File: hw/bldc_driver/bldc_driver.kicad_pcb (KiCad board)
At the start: 2 copper layers, 127.5 x 96 mm, 131 parts, among them J1 430450412, J2 B4B-EH-A(LF)(SN), J3 B4B-EH-A(LF)(SN), J4 1733583, Q1 IRF540N, Q1 Q_NMOS_DGS, Q2 IRF540N, Q3 IRF540N, Q4 IRF540N, Q5 IRF540N, Q6 IRF540N, U1 CH32V30xRxTx, U10 TPS54202DDC, U11 AMC1200BDWV, U12 AMC1200BDWV, U13 AMC1200BDWV, U14 SN65HVD230, U2 STGAP2SCM, U3 STGAP2SCM, U4 STGAP2SCM, U5 STGAP2SCM, U6 STGAP2SCM, U7 STGAP2SCM, U8 TPS54202DDC, U9 AMC1200BDWV

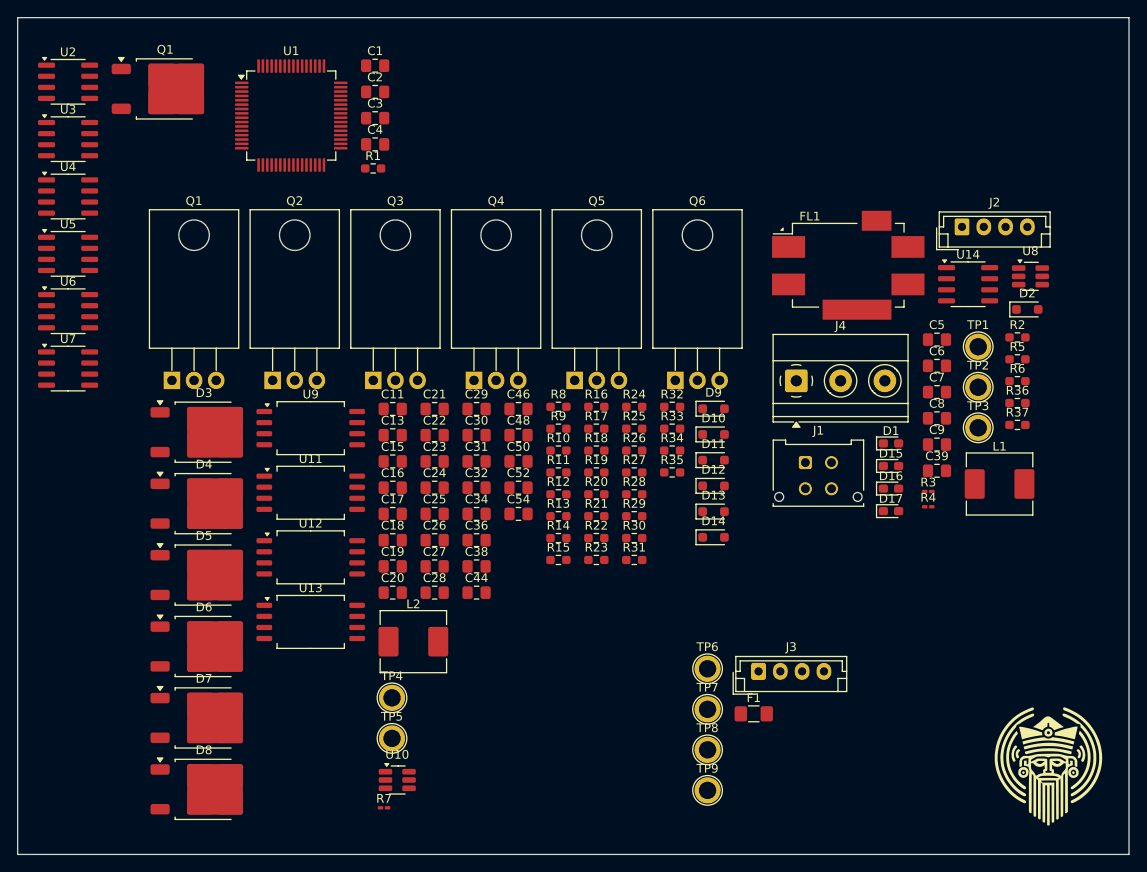
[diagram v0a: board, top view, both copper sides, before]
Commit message: bldc: start placement
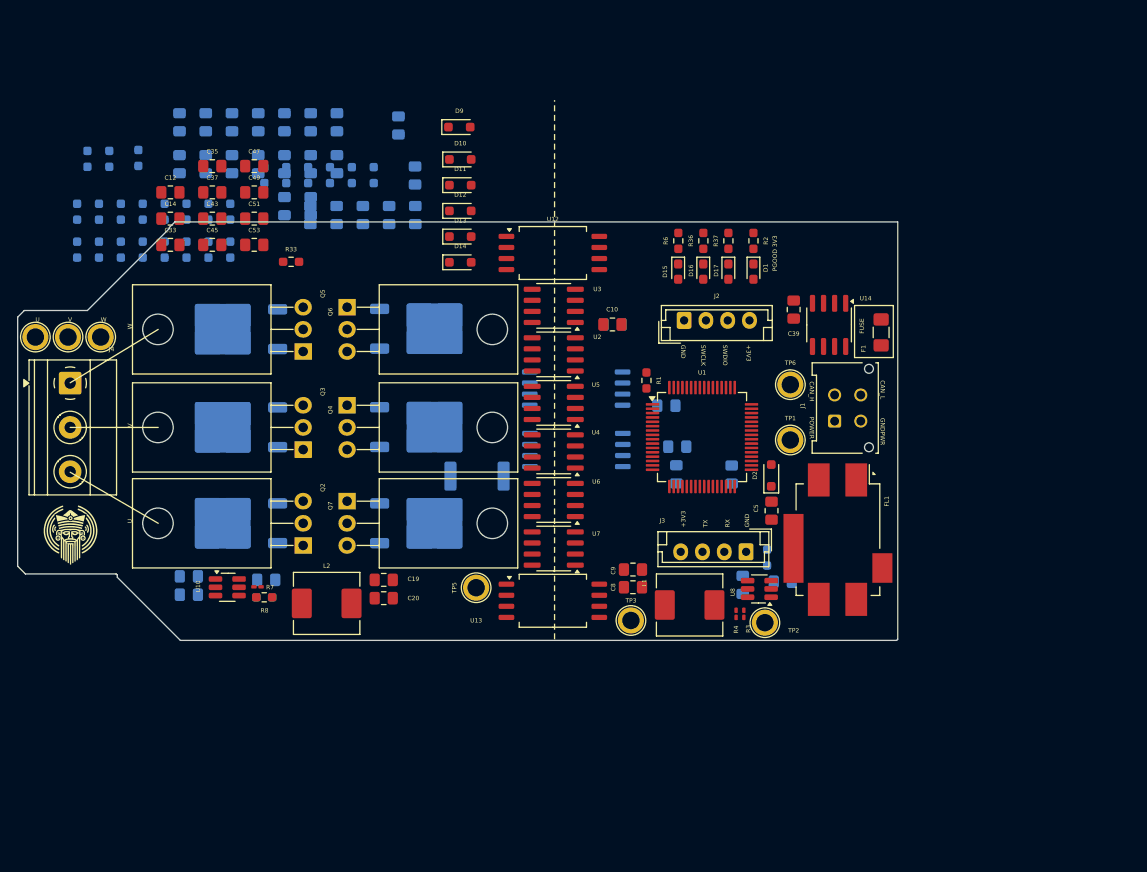
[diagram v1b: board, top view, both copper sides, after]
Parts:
- removed Q1: Q_NMOS_DGS, Package_TO_SOT_SMD:TO-252-2
- removed Q1: IRF540N, Package_TO_SOT_THT:TO-220-3_Horizontal_TabDown
- removed TP4: TestPoint_Flag, TestPoint:TestPoint_Plated_Hole_D2.0mm
- added C10: 1 µF, Capacitor_SMD:C_0805_2012Metric_Pad1.18x1.45mm_HandSolder, F.Cu at (139.7, 79.2)
- added C12: 1 µF, Capacitor_SMD:C_0805_2012Metric_Pad1.18x1.45mm_HandSolder, F.Cu at (89.0, 64.0)
- added C14: 1 µF, Capacitor_SMD:C_0805_2012Metric_Pad1.18x1.45mm_HandSolder, F.Cu at (89.0, 67.1)
- added C33: 1 µF, Capacitor_SMD:C_0805_2012Metric_Pad1.18x1.45mm_HandSolder, F.Cu at (89.0, 70.1)
- added C35: 1 µF, Capacitor_SMD:C_0805_2012Metric_Pad1.18x1.45mm_HandSolder, F.Cu at (93.8, 61.0)
- added C37: 1 µF, Capacitor_SMD:C_0805_2012Metric_Pad1.18x1.45mm_HandSolder, F.Cu at (93.8, 64.0)
- added C43: 1 µF, Capacitor_SMD:C_0805_2012Metric_Pad1.18x1.45mm_HandSolder, F.Cu at (93.8, 67.1)
- added C45: 1 µF, Capacitor_SMD:C_0805_2012Metric_Pad1.18x1.45mm_HandSolder, F.Cu at (93.8, 70.1)
- added C47: 1 µF, Capacitor_SMD:C_0805_2012Metric_Pad1.18x1.45mm_HandSolder, F.Cu at (98.6, 61.0)
- added C49: 1 µF, Capacitor_SMD:C_0805_2012Metric_Pad1.18x1.45mm_HandSolder, F.Cu at (98.6, 64.0)
- added C51: 1 µF, Capacitor_SMD:C_0805_2012Metric_Pad1.18x1.45mm_HandSolder, F.Cu at (98.6, 67.1)
- added C53: 1 µF, Capacitor_SMD:C_0805_2012Metric_Pad1.18x1.45mm_HandSolder, F.Cu at (98.6, 70.1)
- added Q7: IRF540N, Package_TO_SOT_THT:TO-220-3_Horizontal_TabDown, F.Cu at (109.3, 99.5)
- added Rshunt1: HoLLR2512-3W-15mR-1%, Resistor_SMD:R_2512_6332Metric_Pad1.40x3.35mm_HandSolder, B.Cu at (124.2, 96.6)
- C1, C11, C13, C15, C16, C17, C18, C2, C21, C22, C23, C24, C25, C26, C27, C28, C29, C3, C30, C31, C32, C34, C36, C38, C4, C44, C46, C48, C50, C52, C54, C6, C7, D3, D4, D5, D6, D7, D8, R10, R11, R12, R13, R14, R15, R16, R17, R18, R19, R20, R21, R22, R23, R24, R25, R26, R27, R28, R29, R30, R31, R32, R34, R35, R5, R9, U11, U9: moved to B.Cu
- moved TP9 93.0 mm to (73.5, 80.6), turned to 180 degrees
- moved TP8 87.3 mm to (77.3, 80.6)
- moved J4 83.3 mm to (77.5, 85.9), turned to -90 degrees
- moved TP7 81.7 mm to (81.0, 80.6)
- moved R35 76.1 mm to (79.5, 60.2), turned to 90 degrees
- moved R31 75.4 mm to (78.3, 66.3), turned to 90 degrees
- moved R34 72.7 mm to (82.0, 60.2), turned to 90 degrees
- moved R30 71.9 mm to (80.8, 66.3), turned to 90 degrees
- moved R23 69.4 mm to (78.3, 70.6), turned to 90 degrees
- moved R29 68.5 mm to (83.3, 66.3), turned to 90 degrees
- moved R32 67.6 mm to (85.3, 60.1), turned to 90 degrees
- moved R22 66.0 mm to (80.8, 70.6), turned to 90 degrees
- moved R28 65.0 mm to (85.9, 66.3), turned to 90 degrees
- moved U2 63.9 mm to (133.0, 82.6), turned to 180 degrees
- moved U4 62.9 mm to (133.0, 93.8), turned to 180 degrees
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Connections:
- net Net-(J2-Pin_2) renamed /SWCLK
- net Net-(J2-Pin_3) renamed /SWDIO
- J4 pad 1: /Motor/MOTOR_U -> /Motor/MOTOR_W
- J4 pad 3: /Motor/MOTOR_W -> /Motor/MOTOR_U
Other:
- board size 127.5 x 96 mm -> 101 x 48 mm
- copper layers 2 -> 4
- board text added: "+3V3"
- board text added: "CAN_H"
- board text added: "CAN_L"
- board text added: "FUSE"
- board text added: "GND"
- board text added: "GNDPWR"
- board text added: "PGOOD 3V3"
- board text added: "POWER"
- board text added: "RX"
- board text added: "SWCLK"
- board text added: "SWDIO"
- board text added: "TX"
- board text added: "U"
- board text added: "V"
- board text added: "W"
